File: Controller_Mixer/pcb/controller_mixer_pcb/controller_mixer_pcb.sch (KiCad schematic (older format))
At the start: 26 parts, among them J1 Conn_01x08_Male, J10 Conn_01x08_Male, J15 Conn_01x05_Male, J16 Conn_01x05_Male, J17 Conn_01x04_Male, J18 Conn_01x04_Male, J19 Conn_01x08_Male, J2 Conn_01x08_Male, J20 Conn_01x08_Male, J3 Conn_01x08_Male, J4 Conn_01x08_Male, J7 Conn_01x08_Male, J8 Conn_01x08_Male, J9 Conn_01x08_Male, U3 Teensy4.1

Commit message: 1st Controller_Mixer pcb fertig
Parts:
- removed J17, J18, VU-LEDs1, VUs1: Conn_01x04_Male, Connector_PinHeader_2.54mm:PinHeader_1x04_P2.54mm_Vertical, symbol Connector:Conn_01x04_Male
- added J5, J6, VUVs1, VUs1: Conn_01x05_Male, Connector_PinHeader_2.54mm:PinHeader_1x05_P2.54mm_Vertical, symbol Connector:Conn_01x05_Male
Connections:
- wire segments 211 -> 218
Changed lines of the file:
@@
 Wire Wire Line
 	7850 1550 7850 1650
-Connection ~ 7850 1650
 Wire Wire Line
 	4650 700  7150 700
@@
 Text GLabel 7950 2650 1    50   UnSpc ~ 0
 VU-CONNECTORS
-$Comp
-L Connector:Conn_01x04_Male J17
-U 1 1 5FB7A905
-P 7650 2250
-F 0 "J17" H 7758 2531 50  0000 C CNN
-F 1 "Conn_01x04_Male" H 7758 2440 50  0000 C CNN
-F 2 "Connector_PinHeader_2.54mm:PinHeader_1x04_P2.54mm_Vertical" H 7650 2250 50  0001 C CNN
-F 3 "~" H 7650 2250 50  0001 C CNN
-	1    7650 2250
-	1    0    0    -1
-$EndComp
-$Comp
-L Connector:Conn_01x04_Male VUs1
-U 1 1 5FB7E38C
-P 7600 2350
-F 0 "VUs1" H 7572 2232 50  0000 R CNN
-F 1 "Conn_01x04_Male" H 7572 2323 50  0000 R CNN
-F 2 "Connector_PinHeader_2.54mm:PinHeader_1x04_P2.54mm_Vertical" H 7600 2350 50  0001 C CNN
-F 3 "~" H 7600 2350 50  0001 C CNN
-	1    7600 2350
-	-1   0    0    1
-$EndComp
-Connection ~ 7850 2150
-Wire Wire Line
-	7850 2150 7850 2250
-Connection ~ 7850 2250
-Wire Wire Line
-	7850 2250 7850 2350
-Connection ~ 7850 2350
-Wire Wire Line
-	7850 2350 7850 2450
-Connection ~ 7850 2450
-$Comp
-L Connector:Conn_01x04_Male J18
-U 1 1 5FB8B727
-P 7650 3050
-F 0 "J18" H 7758 3331 50  0000 C CNN
-F 1 "Conn_01x04_Male" H 7758 3240 50  0000 C CNN
-F 2 "Connector_PinHeader_2.54mm:PinHeader_1x04_P2.54mm_Vertical" H 7650 3050 50  0001 C CNN
-F 3 "~" H 7650 3050 50  0001 C CNN
-	1    7650 3050
-	1    0    0    -1
-$EndComp
-Wire Wire Line
-	7850 2450 7850 2950
-Connection ~ 7850 2950
-Wire Wire Line
-	7850 2950 7850 3050
-Connection ~ 7850 3050
-Wire Wire Line
-	7850 3050 7850 3150
-Connection ~ 7850 3150
-Wire Wire Line
-	7850 3150 7850 3250
-Connection ~ 7850 3250
-Wire Wire Line
-	7850 3250 7850 3750
 Text GLabel 7950 3250 1    50   UnSpc ~ 0
 VU-LEDS
-Wire Wire Line
-	3750 3250 3750 3650
-Wire Wire Line
-	3750 3650 7150 3650
-Wire Wire Line
-	7150 3650 7150 2150
-Wire Wire Line
-	7150 2150 7400 2150
-Wire Wire Line
-	7400 2250 7100 2250
-Wire Wire Line
-	7100 2250 7100 3600
-Wire Wire Line
-	7100 3600 3850 3600
-Wire Wire Line
-	3850 3600 3850 3250
-Wire Wire Line
-	3950 3250 3950 3550
-Wire Wire Line
-	3950 3550 7050 3550
-Wire Wire Line
-	7050 3550 7050 2350
-Wire Wire Line
-	7050 2350 7400 2350
-Wire Wire Line
-	7400 2450 7000 2450
-Wire Wire Line
-	7000 2450 7000 3500
-Wire Wire Line
-	7000 3500 4050 3500
-Wire Wire Line
-	4050 3500 4050 3250
-Connection ~ 7400 3050
-Wire Wire Line
-	7400 3050 7400 3150
-Connection ~ 7400 3150
-Wire Wire Line
-	7400 3150 7400 3250
-Wire Wire Line
-	7400 3250 6950 3250
-Wire Wire Line
-	6950 3250 6950 3450
-Wire Wire Line
-	6950 3450 4150 3450
-Connection ~ 7400 3250
-Wire Wire Line
-	4150 4000 4300 4000
-Wire Wire Line
-	7400 3000 7400 3050
-Wire Wire Line
-	7400 2950 7400 3050
-Wire Wire Line
-	4150 3250 4150 3450
-Connection ~ 4150 3450
-Wire Wire Line
-	4150 3450 4150 4000
 Connection ~ 4300 4000
 $Comp
@@
 $EndComp
 Wire Wire Line
-	7850 1650 7850 2150
-Wire Wire Line
 	7850 1250 7850 1350
 Connection ~ 7850 1250
@@
 Wire Wire Line
 	7850 1350 7850 1450
-$Comp
-L Connector:Conn_01x04_Male VU-LEDs1
-U 1 1 5FB8B72D
+Wire Wire Line
+	2400 900  2950 900
+Wire Wire Line
+	2950 900  2950 1050
+$Comp
+L Connector:Conn_01x05_Male J5
+U 1 1 5FDC9B36
+P 7650 2350
+F 0 "J5" H 7758 2731 50  0000 C CNN
+F 1 "Conn_01x05_Male" H 7758 2640 50  0000 C CNN
+F 2 "Connector_PinHeader_2.54mm:PinHeader_1x05_P2.54mm_Vertical" H 7650 2350 50  0001 C CNN
+F 3 "~" H 7650 2350 50  0001 C CNN
+	1    7650 2350
+	1    0    0    -1
+$EndComp
+$Comp
+L Connector:Conn_01x05_Male VUs1
+U 1 1 5FDC9B3C
+P 7600 2350
+F 0 "VUs1" H 7572 2282 50  0000 R CNN
+F 1 "Conn_01x05_Male" H 7572 2373 50  0000 R CNN
+F 2 "Connector_PinHeader_2.54mm:PinHeader_1x05_P2.54mm_Vertical" H 7600 2350 50  0001 C CNN
+F 3 "~" H 7600 2350 50  0001 C CNN
+	1    7600 2350
+	-1   0    0    1
+$EndComp
+$Comp
+L Connector:Conn_01x05_Male J6
+U 1 1 5FE2A081
+P 7650 3150
+F 0 "J6" H 7758 3531 50  0000 C CNN
+F 1 "Conn_01x05_Male" H 7758 3440 50  0000 C CNN
+F 2 "Connector_PinHeader_2.54mm:PinHeader_1x05_P2.54mm_Vertical" H 7650 3150 50  0001 C CNN
+F 3 "~" H 7650 3150 50  0001 C CNN
+	1    7650 3150
+	1    0    0    -1
+$EndComp
+$Comp
+L Connector:Conn_01x05_Male VUVs1
+U 1 1 5FE2A087
 P 7600 3150
-F 0 "VU-LEDs1" H 7572 3032 50  0000 R CNN
-F 1 "Conn_01x04_Male" H 7572 3123 50  0000 R CNN
-F 2 "Connector_PinHeader_2.54mm:PinHeader_1x04_P2.54mm_Vertical" H 7600 3150 50  0001 C CNN
+F 0 "VUVs1" H 7572 3082 50  0000 R CNN
+F 1 "Conn_01x05_Male" H 7572 3173 50  0000 R CNN
+F 2 "Connector_PinHeader_2.54mm:PinHeader_1x05_P2.54mm_Vertical" H 7600 3150 50  0001 C CNN
 F 3 "~" H 7600 3150 50  0001 C CNN
 	1    7600 3150
 	-1   0    0    1
 $EndComp
+Wire Wire Line
+	7400 2950 7400 3050
+Connection ~ 7400 3050
+Wire Wire Line
+	7400 3050 7400 3150
+Connection ~ 7400 3150
+Wire Wire Line
+	7400 3150 7400 3250
+Connection ~ 7400 3250
+Wire Wire Line
+	7400 3250 7400 3350
+Connection ~ 7850 3350
+Wire Wire Line
+	7850 3350 7850 3750
+Connection ~ 7850 1650
+Wire Wire Line
+	7850 1650 7850 2150
+Connection ~ 7850 2150
+Wire Wire Line
+	7850 2150 7850 2250
+Connection ~ 7850 2250
+Wire Wire Line
+	7850 2250 7850 2350
+Connection ~ 7850 2350
+Wire Wire Line
+	7850 2350 7850 2450
+Connection ~ 7850 2450
+Wire Wire Line
+	7850 2450 7850 2550
+Connection ~ 7850 2550
+Wire Wire Line
+	7850 2550 7850 2950
+Connection ~ 7850 2950
+Wire Wire Line
+	7850 2950 7850 3050
+Connection ~ 7850 3050
+Wire Wire Line
+	7850 3050 7850 3150
+Connection ~ 7850 3150
+Wire Wire Line
+	7850 3150 7850 3250
+Connection ~ 7850 3250
+Wire Wire Line
+	7850 3250 7850 3350
+Connection ~ 7400 3350
+Wire Wire Line
+	2400 900  2400 4000
+Wire Wire Line
+	2400 4000 4300 4000
+Wire Wire Line
+	4150 3250 4150 3650
+Wire Wire Line
+	4150 3650 7400 3650
+Wire Wire Line
+	7400 3350 7400 3650
+Wire Wire Line
+	4050 3250 4050 3600
+Wire Wire Line
+	4050 3600 7300 3600
+Wire Wire Line
+	7300 3600 7300 2550
+Wire Wire Line
+	7300 2550 7400 2550
+Wire Wire Line
+	7400 2450 7250 2450
+Wire Wire Line
+	7250 2450 7250 3550
+Wire Wire Line
+	7250 3550 3950 3550
+Wire Wire Line
+	3950 3550 3950 3250
+Wire Wire Line
+	3850 3250 3850 3500
+Wire Wire Line
+	3850 3500 7150 3500
+Wire Wire Line
+	7150 3500 7150 2350
+Wire Wire Line
+	7150 2350 7400 2350
+Wire Wire Line
+	7400 2250 7100 2250
+Wire Wire Line
+	7100 2250 7100 3450
+Wire Wire Line
+	7100 3450 3750 3450
+Wire Wire Line
+	3750 3450 3750 3250
+Wire Wire Line
+	3650 3250 3650 3400
+Wire Wire Line
+	3650 3400 7050 3400
+Wire Wire Line
+	7050 3400 7050 2150
+Wire Wire Line
+	7050 2150 7400 2150
 $EndSCHEMATC

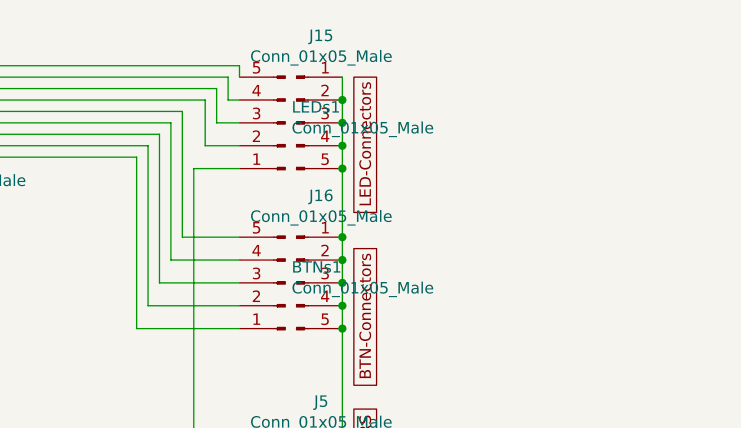
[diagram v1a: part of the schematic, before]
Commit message: 1st Controller_Mixer pcb fertig
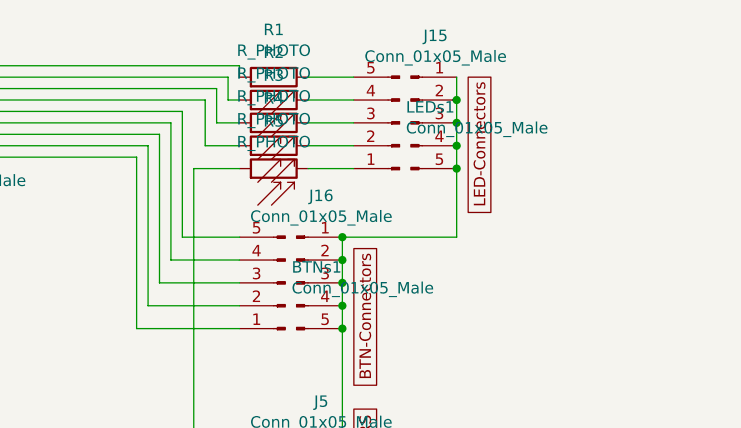
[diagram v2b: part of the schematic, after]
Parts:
- added R1, R2, R3, R4, R5: R_PHOTO, Resistor_THT:R_Axial_DIN0207_L6.3mm_D2.5mm_P5.08mm_Vertical, symbol Device:R_PHOTO
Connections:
- net at U3.16 (24_A10_TX6_SCL2): now also R5.1; no longer LEDs1.1 (Pin_1)
- net at U3.30 (38_CS1_IN1): now also R4.1; no longer LEDs1.2 (Pin_2)
- net at U3.31 (39_MISO1_OUT1A): now also R3.1; no longer LEDs1.3 (Pin_3)
- net at U3.32 (40_A16): now also R2.1; no longer LEDs1.4 (Pin_4)
- net at U3.33 (41_A17): now also R1.1; no longer LEDs1.5 (Pin_5)
- new net: LEDs1.5 (Pin_5), R1.2
- new net: LEDs1.4 (Pin_4), R2.2
- new net: LEDs1.3 (Pin_3), R3.2
- new net: LEDs1.2 (Pin_2), R4.2
- new net: LEDs1.1 (Pin_1), R5.2
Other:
- moved on the sheet: J15, LEDs1
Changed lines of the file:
@@
 Wire Wire Line
 	1950 5600 1950 700
-Text GLabel 7950 550  3    50   UnSpc ~ 0
+Text GLabel 8450 550  3    50   UnSpc ~ 0
 LED-Connectors
 Text GLabel 7950 1300 3    50   UnSpc ~ 0
@@
 	7350 550  7350 650
 Wire Wire Line
-	7350 650  7400 650
-Wire Wire Line
 	4450 600  7300 600
 Wire Wire Line
 	7300 600  7300 750
 Wire Wire Line
-	7300 750  7400 750
-Wire Wire Line
 	4550 650  7250 650
 Wire Wire Line
 	7250 650  7250 850
 Wire Wire Line
-	7250 850  7400 850
-Wire Wire Line
 	7200 3700 7200 950
 Wire Wire Line
-	7200 950  7400 950
+	7700 950  7900 950
 Wire Wire Line
 	4250 3700 7200 3700
 Wire Wire Line
-	7850 550  7850 650
-Connection ~ 7850 650
-Wire Wire Line
-	7850 650  7850 750
-Connection ~ 7850 750
-Wire Wire Line
-	7850 750  7850 850
-Connection ~ 7850 850
-Wire Wire Line
-	7850 850  7850 950
-Connection ~ 7850 950
+	8350 550  8350 650
+Connection ~ 8350 650
+Wire Wire Line
+	8350 650  8350 750
+Connection ~ 8350 750
+Wire Wire Line
+	8350 750  8350 850
+Connection ~ 8350 850
+Wire Wire Line
+	8350 850  8350 950
+Connection ~ 8350 950
 Connection ~ 7850 1450
 Wire Wire Line
@@
 L Connector:Conn_01x05_Male J15
 U 1 1 5FA665C1
-P 7650 750
-F 0 "J15" H 7758 1131 50  0000 C CNN
-F 1 "Conn_01x05_Male" H 7758 1040 50  0000 C CNN
-F 2 "Connector_PinHeader_2.54mm:PinHeader_1x05_P2.54mm_Vertical" H 7650 750 50  0001 C CNN
-F 3 "~" H 7650 750 50  0001 C CNN
-	1    7650 750
+P 8150 750
+F 0 "J15" H 8258 1131 50  0000 C CNN
+F 1 "Conn_01x05_Male" H 8258 1040 50  0000 C CNN
+F 2 "Connector_PinHeader_2.54mm:PinHeader_1x05_P2.54mm_Vertical" H 8150 750 50  0001 C CNN
+F 3 "~" H 8150 750 50  0001 C CNN
+	1    8150 750
 	1    0    0    -1
 $EndComp
 Wire Wire Line
-	7850 950  7850 1250
+	8350 950  8350 1250
 $Comp
 L Connector:Conn_01x05_Male LEDs1
 U 1 1 5FA69E13
-P 7600 750
-F 0 "LEDs1" H 7572 682 50  0000 R CNN
-F 1 "Conn_01x05_Male" H 7572 773 50  0000 R CNN
-F 2 "Connector_PinHeader_2.54mm:PinHeader_1x05_P2.54mm_Vertical" H 7600 750 50  0001 C CNN
-F 3 "~" H 7600 750 50  0001 C CNN
-	1    7600 750
+P 8100 750
+F 0 "LEDs1" H 8072 682 50  0000 R CNN
+F 1 "Conn_01x05_Male" H 8072 773 50  0000 R CNN
+F 2 "Connector_PinHeader_2.54mm:PinHeader_1x05_P2.54mm_Vertical" H 8100 750 50  0001 C CNN
+F 3 "~" H 8100 750 50  0001 C CNN
+	1    8100 750
 	-1   0    0    1
 $EndComp
 Wire Wire Line
 	7850 1250 7850 1350
-Connection ~ 7850 1250
 Connection ~ 7850 1350
 Wire Wire Line
@@
 Wire Wire Line
 	7050 2150 7400 2150
+$Comp
+L Device:R_PHOTO R1
+U 1 1 5F92DF7D
+P 7550 550
+F 0 "R1" V 7757 550 50  0000 C CNN
+F 1 "R_PHOTO" V 7666 550 50  0000 C CNN
+F 2 "Resistor_THT:R_Axial_DIN0207_L6.3mm_D2.5mm_P5.08mm_Vertical" V 7600 300 50  0001 L CNN
+F 3 "~" H 7550 500 50  0001 C CNN
+	1    7550 550
+	0    -1   -1   0
+$EndComp
+$Comp
+L Device:R_PHOTO R2
+U 1 1 5F96E19E
+P 7550 650
+F 0 "R2" V 7757 650 50  0000 C CNN
+F 1 "R_PHOTO" V 7666 650 50  0000 C CNN
+F 2 "Resistor_THT:R_Axial_DIN0207_L6.3mm_D2.5mm_P5.08mm_Vertical" V 7600 400 50  0001 L CNN
+F 3 "~" H 7550 600 50  0001 C CNN
+	1    7550 650
+	0    -1   -1   0
+$EndComp
+$Comp
+L Device:R_PHOTO R3
+U 1 1 5F97B054
+P 7550 750
+F 0 "R3" V 7757 750 50  0000 C CNN
+F 1 "R_PHOTO" V 7666 750 50  0000 C CNN
+F 2 "Resistor_THT:R_Axial_DIN0207_L6.3mm_D2.5mm_P5.08mm_Vertical" V 7600 500 50  0001 L CNN
+F 3 "~" H 7550 700 50  0001 C CNN
+	1    7550 750
+	0    -1   -1   0
+$EndComp
+$Comp
+L Device:R_PHOTO R4
+U 1 1 5F987FB9
+P 7550 850
+F 0 "R4" V 7757 850 50  0000 C CNN
+F 1 "R_PHOTO" V 7666 850 50  0000 C CNN
+F 2 "Resistor_THT:R_Axial_DIN0207_L6.3mm_D2.5mm_P5.08mm_Vertical" V 7600 600 50  0001 L CNN
+F 3 "~" H 7550 800 50  0001 C CNN
+	1    7550 850
+	0    -1   -1   0
+$EndComp
+$Comp
+L Device:R_PHOTO R5
+U 1 1 5F994DBD
+P 7550 950
+F 0 "R5" V 7757 950 50  0000 C CNN
+F 1 "R_PHOTO" V 7666 950 50  0000 C CNN
+F 2 "Resistor_THT:R_Axial_DIN0207_L6.3mm_D2.5mm_P5.08mm_Vertical" V 7600 700 50  0001 L CNN
+F 3 "~" H 7550 900 50  0001 C CNN
+	1    7550 950
+	0    -1   -1   0
+$EndComp
+Wire Wire Line
+	7350 650  7400 650
+Wire Wire Line
+	7300 750  7400 750
+Wire Wire Line
+	7250 850  7400 850
+Wire Wire Line
+	7200 950  7400 950
+Wire Wire Line
+	7700 850  7900 850
+Wire Wire Line
+	7700 750  7900 750
+Wire Wire Line
+	7700 650  7900 650
+Wire Wire Line
+	7700 550  7900 550
+Wire Wire Line
+	7850 1250 8350 1250
+Connection ~ 7850 1250
 $EndSCHEMATC
